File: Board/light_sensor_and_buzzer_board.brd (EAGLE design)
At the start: 35 x 27.4 mm, 5 parts, among them U1 TEM-HUM-AM2302(4P-25.0X15.0MM)

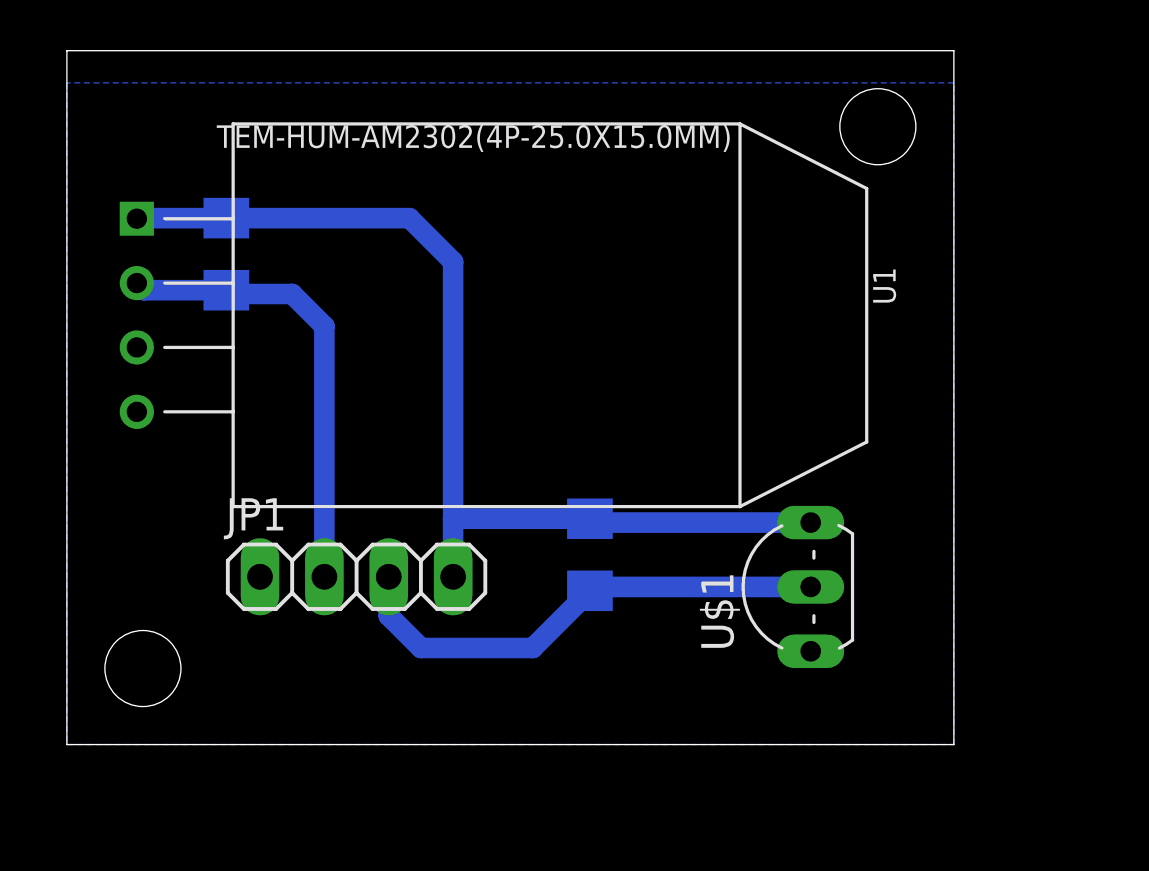
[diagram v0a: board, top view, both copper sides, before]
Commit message: Update
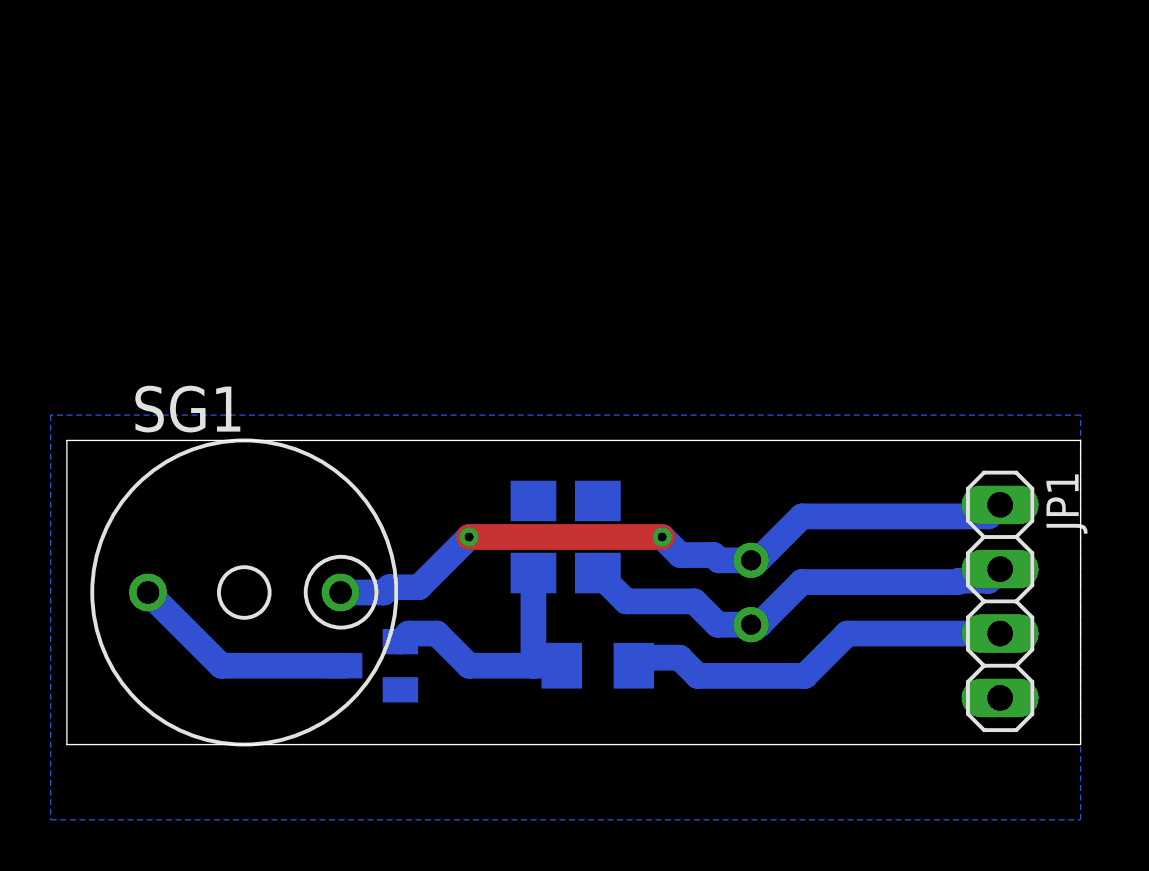
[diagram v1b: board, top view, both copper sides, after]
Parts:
- removed U$1: DS18B20, DS18B20_PAR:TO92-
- added OPH1: 5-10k, photo-elements:VT900
- added R3: 100k, rcl:R1206
- added SG1: BMT1205XH7.5, buzzer:BMT1205XH7.5
- R1: value (none) -> 10k
- R2: value (none) -> 470
- U1: value TEM-HUM-AM2302(4P-25.0X15.0MM) -> IRLML2502; device TEM-HUM-AM2302_4P-25.0X15.0MM_:SNR4-2.54-25.0X15.0X7.0MM -> IRLML2502TRPBF:SOT23
- moved JP1 25.4 mm to (36.8, 5.65), turned to 270 degrees
- moved R2 21.9 mm to (20.9, 3.11), turned to 180 degrees
- moved U1 14.5 mm to (12.1, 3.11), flipped to the bottom
- moved R1 0.77 mm to (20.9, 8.19), turned to 270 degrees
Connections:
- new net N$3: R2.1, R3.2, U1.1
- new net N$4: JP1.3, R2.2
- net +3V3: now also JP1.1, OPH1.1, SG1.+; no longer JP1.4, R1.2, R2.2, U$1.1, U1.P$1
- net GND: now also JP1.4, R1.1, R3.1, U1.2; no longer JP1.1, U$1.3, U1.P$4
- net N$1: now also OPH1.2, R1.2; no longer R2.1, U1.P$2
- net N$2: now also SG1.-, U1.3; no longer JP1.3, R1.1, U$1.2
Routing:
- net N$4: track 0.00 -> 15.6 mm
- net +3V3: track 40.2 -> 28.2 mm, vias 0 -> 2
- net N$2: track 19.7 -> 8.96 mm
- net N$3: track 0.00 -> 10.7 mm
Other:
- board size 35 x 27.4 mm -> 40 x 12 mm
